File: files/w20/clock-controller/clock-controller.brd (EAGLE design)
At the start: 23.8 x 55.7 mm, 16 parts

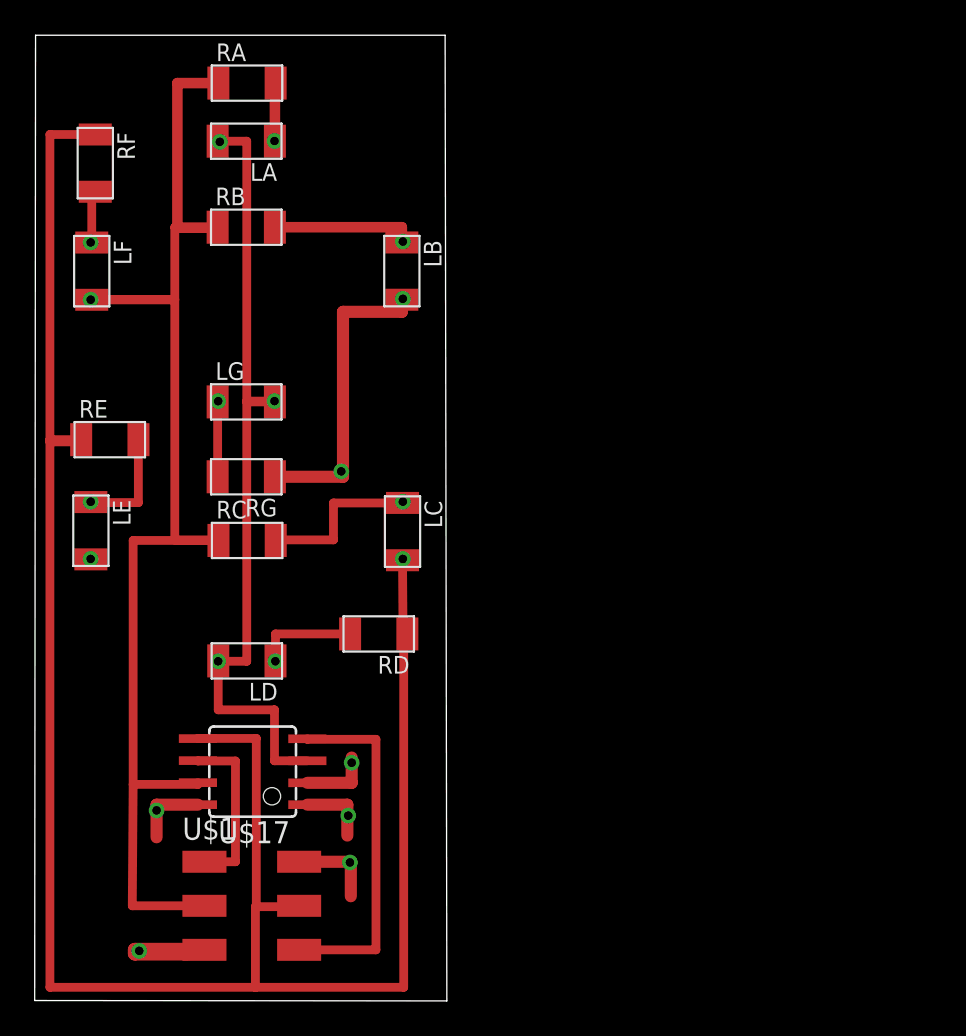
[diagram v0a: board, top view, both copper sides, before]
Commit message: board production
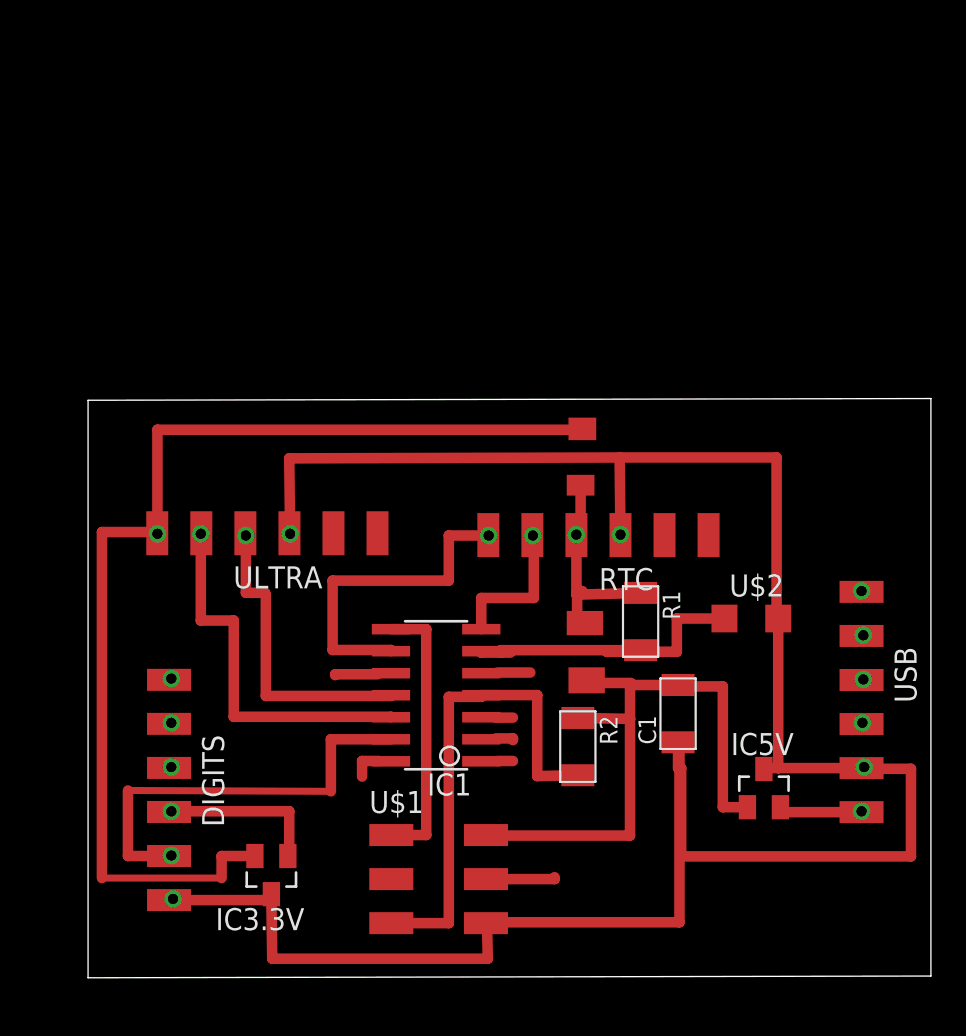
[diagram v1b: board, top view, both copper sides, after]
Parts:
- removed LA, LB, LC, LD, LE, LF, LG: LEDFAB1206, fab:LED1206FAB
- removed RA, RB, RC, RD, RE, RF, RG: (no value), fab:R1206FAB
- removed U$17: ATTINY45SI, fab:SOIC8
- added C1: CAP-US1206FAB, fab:C1206FAB
- added DIGITS, RTC, ULTRA, USB: FTDI-SMD-HEADER, fab:1X06SMD
- added IC1: ATTINY44-SSU, fab:SOIC14
- added IC3.3V, IC5V: (no value), fab:SOT23
- added R1: 49.9K, fab:R1206FAB
- added R2: 10K, fab:R1206FAB
- added U$2: PHOTOTRANSISTOR-NPN1206, fab:OP1206
- moved U$1 10.9 mm to (23.3, 7.29)
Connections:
- removed net MOSI: LC.2, RD.1, RE.1, RF.1, U$1.4, U$17.5
- removed net N$1: LA.1, RA.2
- removed net N$2: LB.1, RB.2
- removed net N$3: LC.1, RC.2
- removed net N$4: LD.1, RD.2
- removed net N$5: LE.1, RE.2
- removed net N$6: LF.1, RF.2
- removed net N$7: LG.1, RG.2
- removed net PB3: LB.2, LE.2, RG.1, U$17.2
- removed net PB4: LA.2, LD.2, LG.2, U$17.3
- new net ECHO: IC1.11, ULTRA.3
- new net PT: IC1.6, R1.2, U$2.COLLECTOR
- new net SBUS: DIGITS.2, IC1.13
- new net SCL: IC1.9, RTC.1
- new net SDA: IC1.7, RTC.2, U$1.4
- new net TRIG: IC1.12, ULTRA.2
- new net VCC33: DIGITS.3, IC3.3V.1
- new net VIN: IC5V.2, USB.1
- net GND: now also C1.1, DIGITS.1, IC1.14, IC3.3V.3, IC5V.3, RTC.4, U$2.EMITTER, ULTRA.4, USB.2; no longer U$17.4
- net MISO: now also IC1.8; no longer U$17.6
- net RST: now also IC1.4, R2.2; no longer U$17.1
- net SCK: no longer LF.2, RA.1, RB.1, RC.1, U$17.7
- net VCC: now also C1.2, IC1.1, IC3.3V.2, IC5V.1, R1.1, R2.1, RTC.3, ULTRA.1; no longer U$17.8
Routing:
- net MOSI: track 121.5 -> 0.00 mm
- net GND: track 20.6 -> 134.4 mm
- net SCK: track 79.7 -> 0.00 mm
- net VCC: track 9.24 -> 74.3 mm
- net PB4: track 47.5 -> 0.00 mm, vias 1 -> 0
- net SBUS: track 0.00 -> 24.3 mm
- net TRIG: track 0.00 -> 21.6 mm, vias 0 -> 1
- net PB3: track 21.5 -> 0.00 mm
- net N$3: track 9.99 -> 30.6 mm, vias 0 -> 1
- net PT: track 0.00 -> 20.6 mm
- net SCL: track 0.00 -> 19.3 mm, vias 0 -> 1
- net ECHO: track 0.00 -> 17.8 mm, vias 0 -> 1
- net RST: track 11.3 -> 28.6 mm
- net SDA: track 0.00 -> 12.6 mm
- net VCC33: track 0.00 -> 9.63 mm, vias 0 -> 1
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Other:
- board size 23.8 x 55.7 mm -> 48.6 x 33.4 mm

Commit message: fix boards
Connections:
- removed net SCK: U$1.3
- net SCL: now also U$1.3
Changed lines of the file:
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@@
 <wire x1="25.9735" y1="17.8" x2="25.9735" y2="17.89" width="0.6096" layer="1"/>
-</signal>
-<signal name="SCK">
-<contactref element="U$1" pad="3"/>
 </signal>
 <signal name="MISO">
@@
 <wire x1="20.7665" y1="20.5" x2="20.7665" y2="20.43" width="0.6096" layer="1"/>
 <via x="26.4" y="27.1" extent="1-16" drill="0.6" shape="square"/>
+<contactref element="U$1" pad="3"/>
+<wire x1="20.785" y1="7.29" x2="20.7665" y2="20.43" width="0" layer="19" extent="1-1"/>
 </signal>
 <signal name="PT">
